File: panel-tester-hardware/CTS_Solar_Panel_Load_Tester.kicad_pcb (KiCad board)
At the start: 2 copper layers, 50 x 42.5 mm, 11 parts, among them J1 Screw_Terminal_01x02, J2 Conn_01x02_Pin, J3 Conn_01x07, U1 INA219AxD

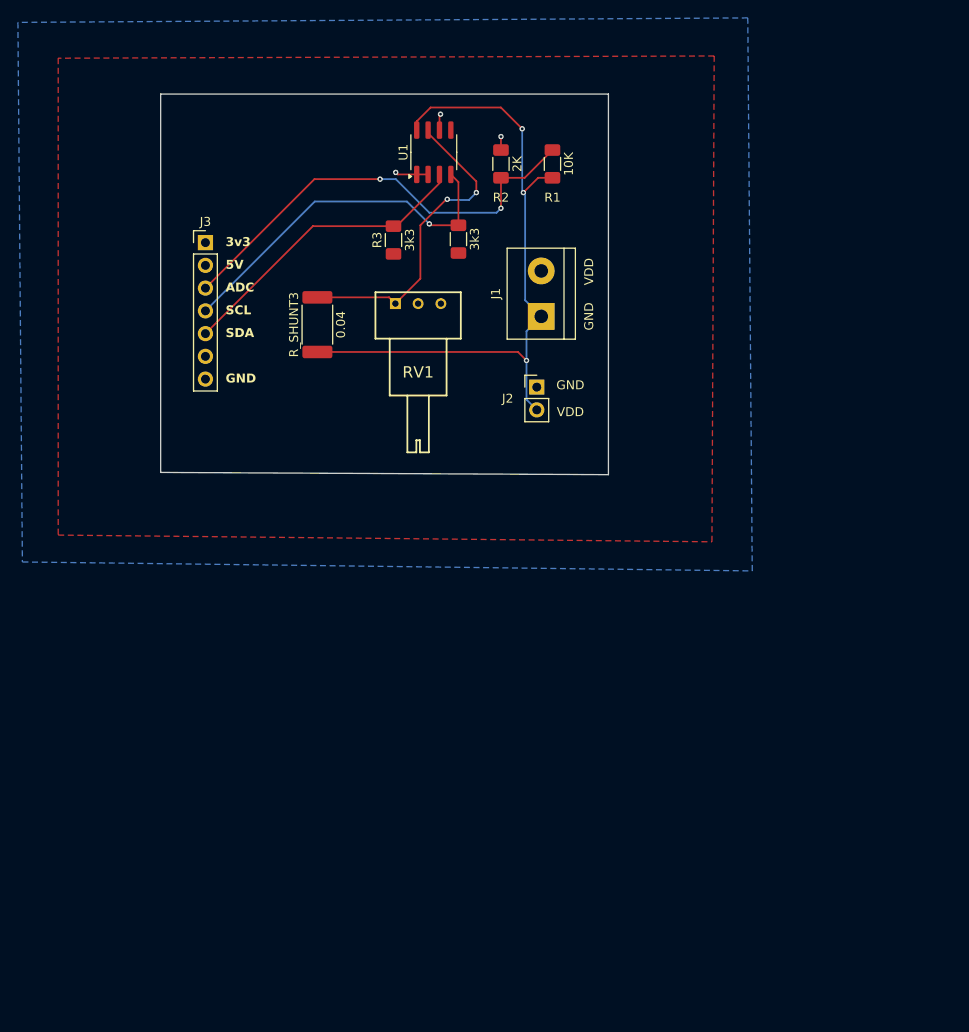
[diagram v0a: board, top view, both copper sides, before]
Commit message: Bluepill layout edits
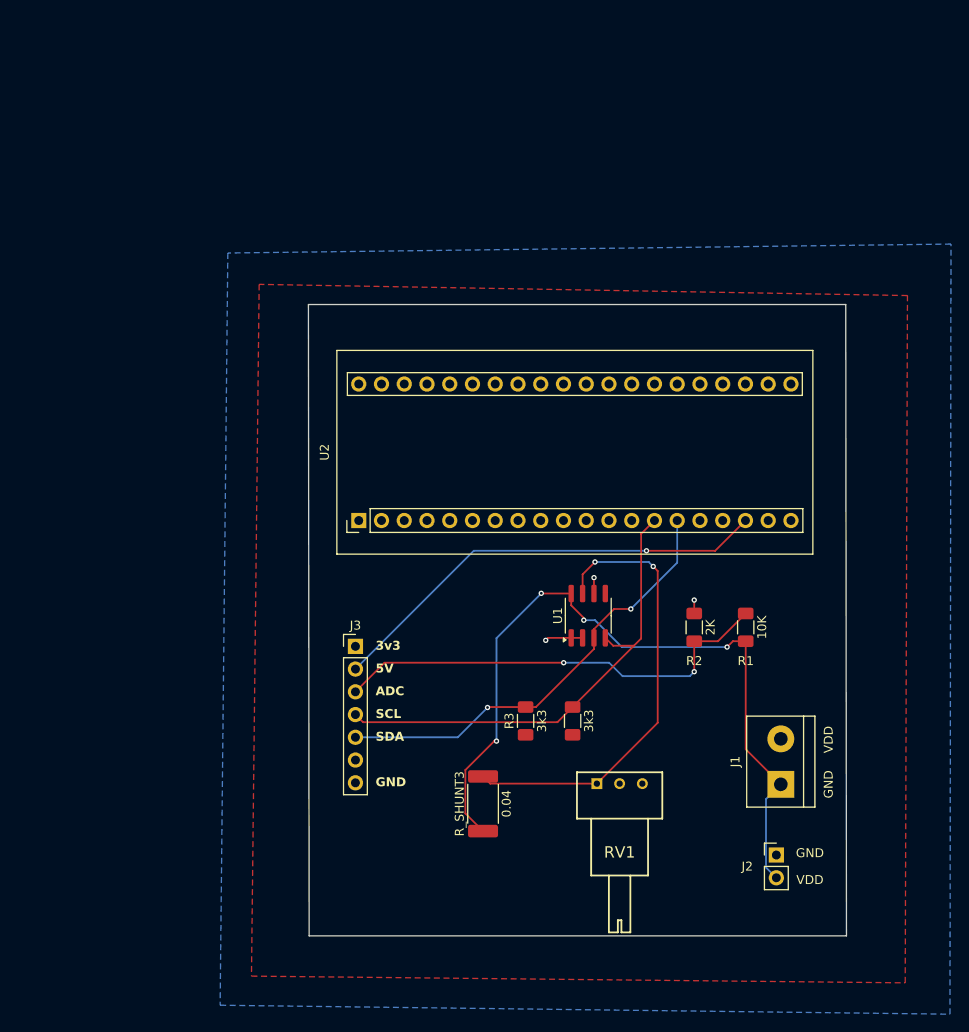
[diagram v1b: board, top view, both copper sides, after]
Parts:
- added U2: YAAJ_BluePill, BluePill:YAAJ_BluePill_2, F.Cu at (97.1, 80.1)
- moved J1 58.7 mm to (144.2, 109.6)
- moved J2 58.7 mm to (143.8, 117.5)
- moved RV1 58.1 mm to (123.7, 109.5)
- moved R_SHUNT3 56.6 mm to (111.0, 111.8)
- moved R1 56.1 mm to (140.3, 92.0)
- moved R2 56.1 mm to (134.6, 92.0)
- moved R3 55.7 mm to (115.8, 102.5)
- moved R4 55.3 mm to (121.0, 102.5)
- moved U1 54.5 mm to (122.8, 90.8)
- moved J3 48.1 mm to (96.8, 94.2)
- moved G*** 31.3 mm to (104.8, 59.5)
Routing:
- net +5V: track 0.00 -> 50.9 mm, vias 0 -> 1
- net MCU_I2C_SDA: track 34.1 -> 50.0 mm, vias 0 -> 2
- net Net-(U1-IN-): track 35.9 -> 51.1 mm
- net MCU_I2C_SCL: track 40.4 -> 53.5 mm, vias 1 -> 0
- net V_SOLAR_INPUT_POS: track 75.6 -> 86.7 mm, vias 3 -> 4
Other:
- board size 50 x 42.5 mm -> 60.1 x 70.5 mm
